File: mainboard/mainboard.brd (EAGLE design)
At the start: 100 x 61 mm, 27 parts, among them J1 BATTERY_CONNDEANS, P1 IMU, P2 analogin, P3 analogin, P4 I2C, U1 DWM1000, U2 ESP8266, X1 04-JST-B4B-XH-A, X2 04-JST-B4B-XH-A

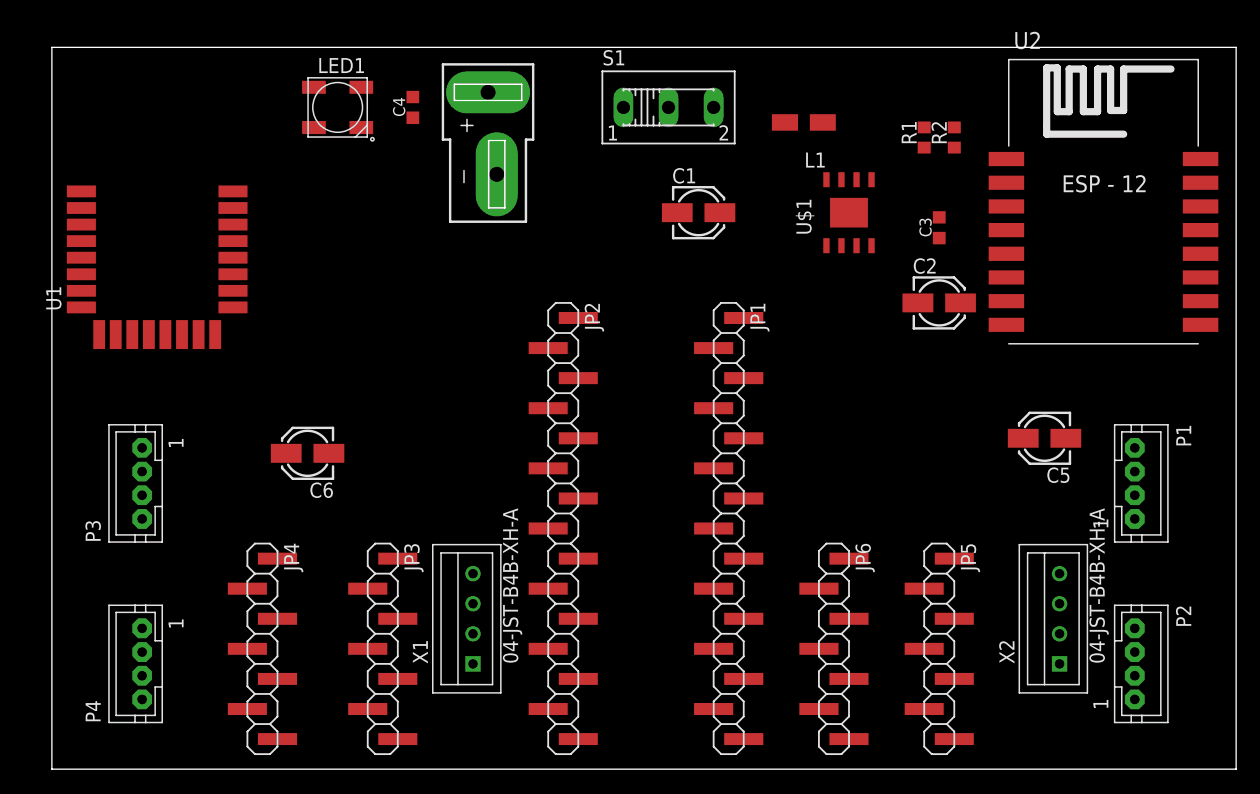
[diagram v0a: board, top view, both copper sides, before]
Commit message: fit
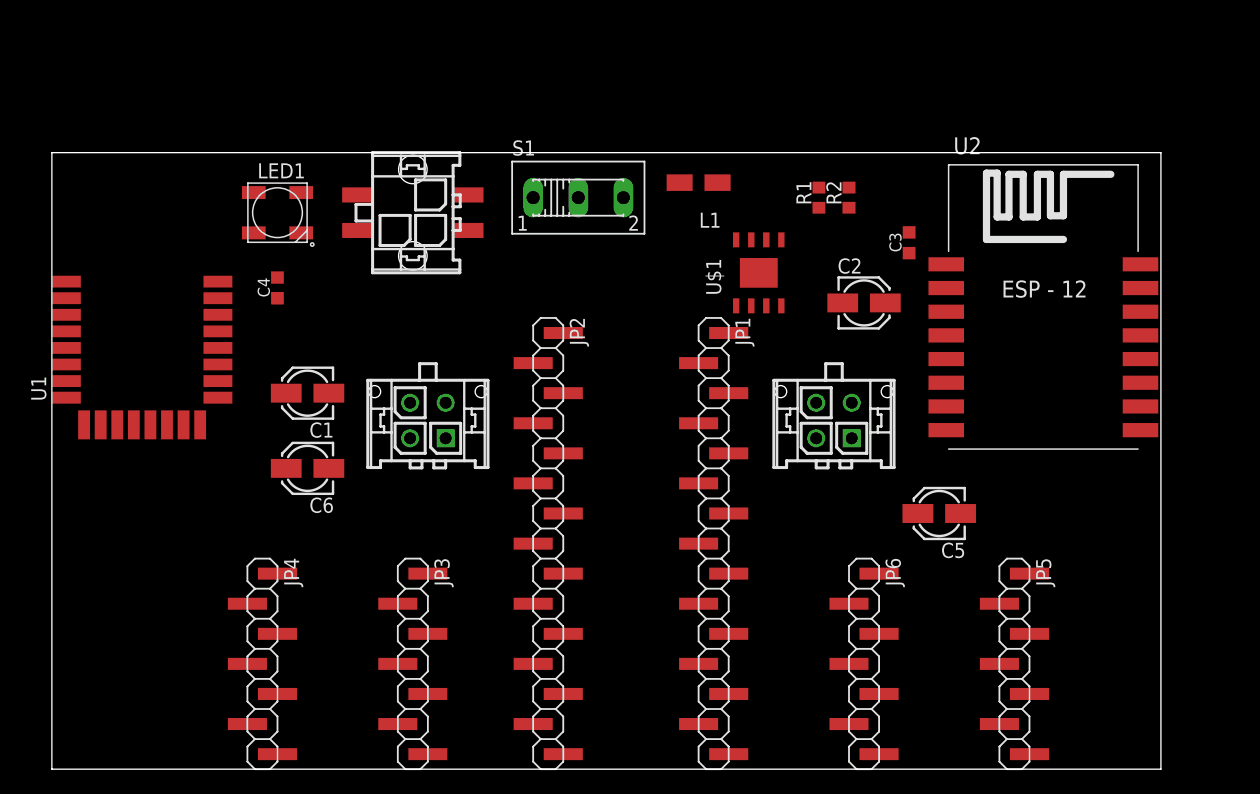
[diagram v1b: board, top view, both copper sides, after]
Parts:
- removed J1: BATTERY_CONNDEANS, SparkFun-Connectors:DEANS
- removed P1: IMU, jst-ph:JST-PH4
- removed P2, P3: analogin, jst-ph:JST-PH4
- removed P4: I2C, jst-ph:JST-PH4
- added X3: (no value), con-molex-micro-fit-3_0:43045-0415
- X1, X2: value 04-JST-B4B-XH-A -> (none); device bt_con-jst-xh:B4B-XH -> con-molex-micro-fit-3_0:43045-0412
- moved C1 36.4 mm to (21.6, 31.8), turned to 180 degrees
- moved X2 24.4 mm to (66.0, 27.9), turned to 0 degrees
- moved C4 19.1 mm to (19.1, 40.6)
- moved X1 15.7 mm to (31.8, 27.9), turned to 0 degrees
- moved C5 10.9 mm to (74.9, 21.6)
- moved S1 10.8 mm to (44.5, 48.3)
- moved U2 10.2 mm to (83.8, 36.8)
- moved R1 10.2 mm to (64.8, 48.3)
- moved R2 10.2 mm to (67.3, 48.3)
- moved L1 10.2 mm to (54.6, 49.5)
- moved LED1 10.2 mm to (19.1, 47.0)
- moved U$1 9.16 mm to (59.7, 41.9)
- moved U1 7.73 mm to (7.62, 39.4)
- moved JP5 6.48 mm to (81.3, 15.2)
- moved C2 6.35 mm to (68.6, 39.4)
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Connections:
- removed net N$1: P1.3
- removed net N$10: P3.3
- removed net N$11: P3.2
- removed net N$12: P3.1
- removed net N$13: P4.3
- removed net N$14: P4.2
- removed net N$15: P4.1
- removed net N$3: P1.2
- removed net N$6: P1.1
- removed net N$7: P2.3
- removed net N$8: P2.2
- removed net N$9: P2.1
- net +12V: now also X3.P$3, X3.P$4; no longer J1.+
- net GND: now also X3.P$1, X3.P$2; no longer P1.4, P2.4, P3.4, P4.4
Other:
- board size 100 x 61 mm -> 93.7 x 52.1 mm
